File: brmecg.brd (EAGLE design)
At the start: 60.6 x 28.6 mm, 42 parts, among them U1 ADS1194CPAG

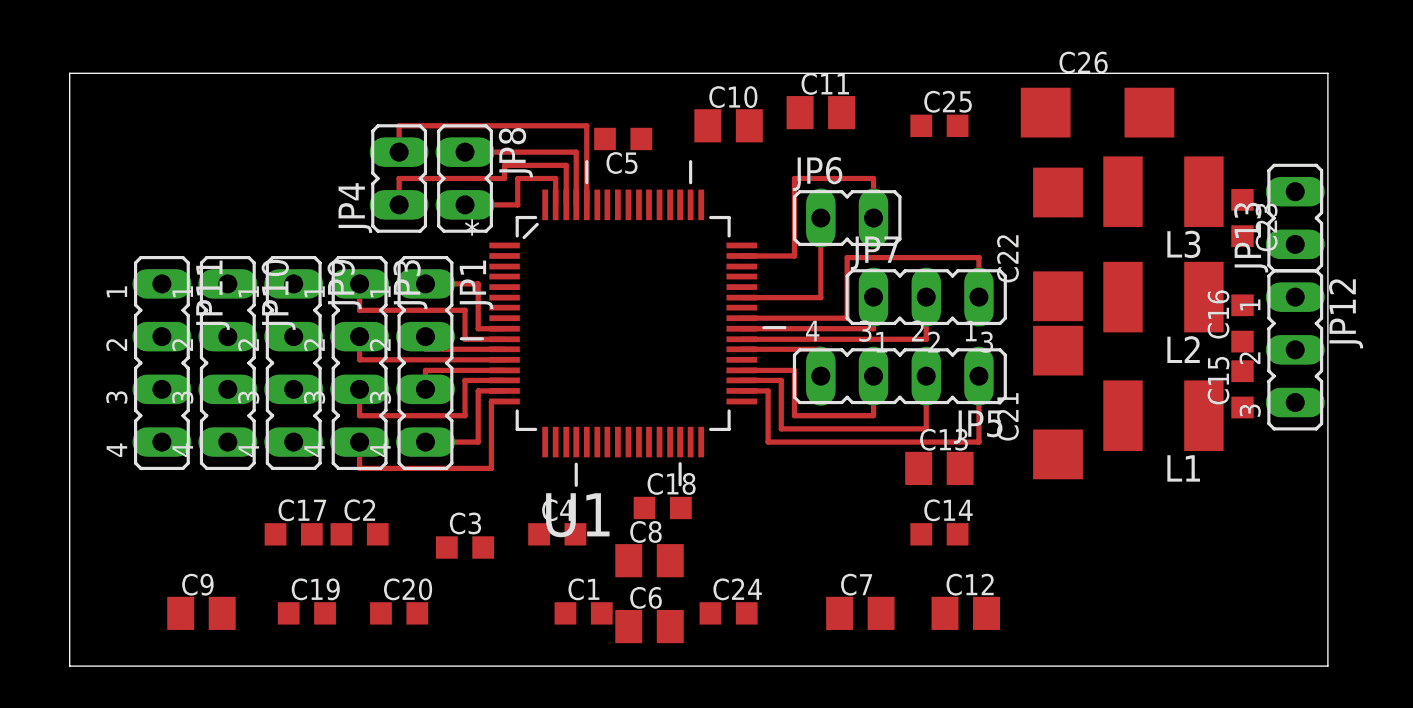
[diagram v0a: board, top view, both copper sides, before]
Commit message: Prepared for sex
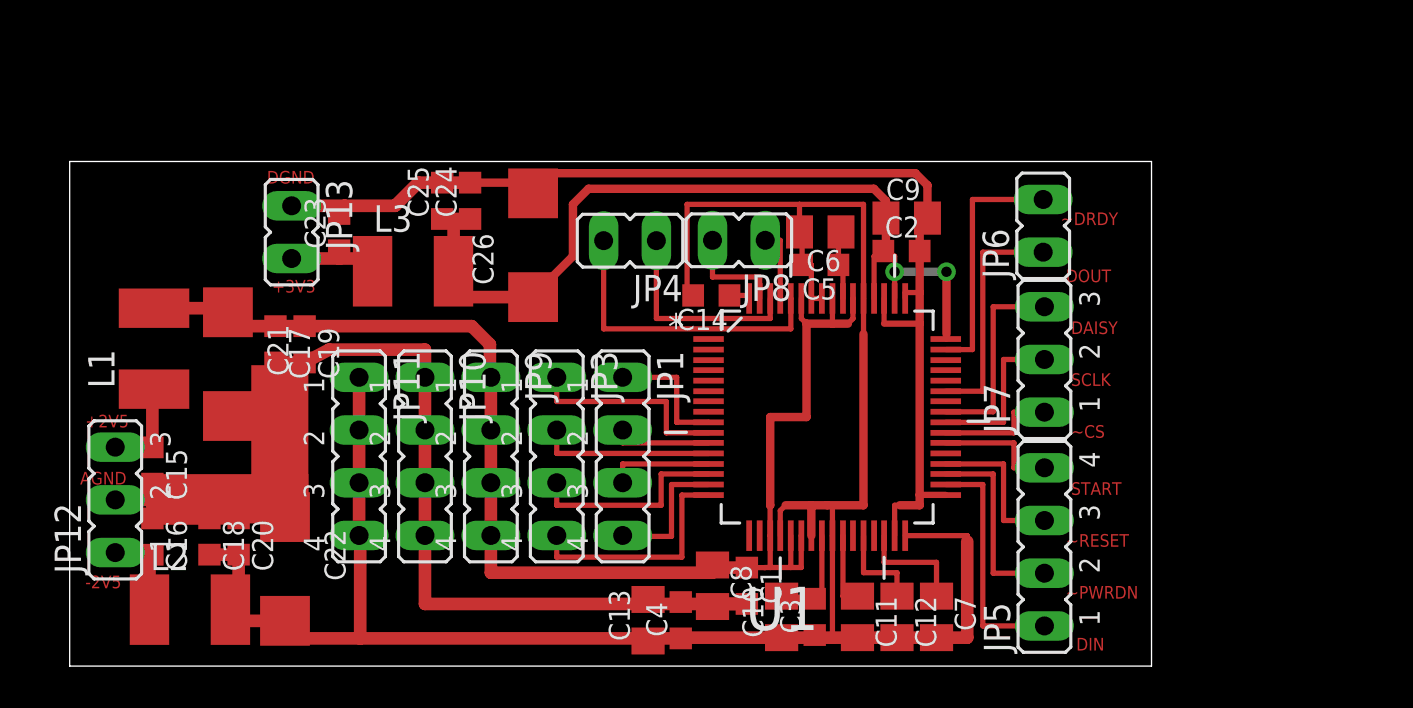
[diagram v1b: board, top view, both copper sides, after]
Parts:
- moved JP12 57.3 mm to (2.19, 8.01), turned to 90 degrees
- moved C16 53.5 mm to (3.98, 6.24), turned to 270 degrees
- moved C15 52.7 mm to (3.98, 9.66), turned to 270 degrees
- moved L2 49.3 mm to (5.79, 2.72), turned to 0 degrees
- moved L1 48.7 mm to (4.07, 15.3), turned to 90 degrees
- moved JP13 48.4 mm to (10.7, 20.9), turned to 180 degrees
- moved C23 43.5 mm to (13.0, 20.9), turned to 90 degrees
- moved C22 40.4 mm to (10.4, 4.68), turned to 270 degrees
- moved C21 40.0 mm to (7.62, 14.6), turned to 270 degrees
- moved C9 39.0 mm to (40.3, 21.6)
- moved L3 36.4 mm to (16.5, 19.0), turned to 0 degrees
- moved C2 29.5 mm to (40.1, 20.0)
- moved C26 27.9 mm to (22.3, 20.3), turned to 90 degrees
- moved C11 24.4 mm to (38.0, 2.37), turned to 270 degrees
- moved C25 24.2 mm to (17.9, 22.4), turned to 90 degrees
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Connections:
- net N$18 renamed DIN
- net N$19 renamed ~PWDN
- net N$20 renamed ~RESET
- net N$21 renamed START
- net N$23 renamed DAISY_IN
- net N$26 renamed DOUT
- net N$27 renamed ~DRDY
- removed net N$22: JP7.1, U1.40
- removed net N$25: JP7.2, U1.39
- new net SCLK: JP7.2, U1.40
- new net ~CS: JP7.1, U1.39
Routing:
- net -2V5: track 0.00 -> 109.4 mm
- net +2V5: track 0.00 -> 66.3 mm
- net AGND: track 0.00 -> 57.0 mm
- net GND: track 0.00 -> 56.7 mm
- net +3V3: track 0.00 -> 43.7 mm, vias 0 -> 2
- net N$25: track 10.9 -> 0.00 mm
- net N$22: track 7.87 -> 0.00 mm
- net SCLK: track 0.00 -> 7.78 mm
- net DAISY_IN: track 16.3 -> 9.82 mm
- net ~CS: track 0.00 -> 5.75 mm
- net DIN: track 17.1 -> 11.6 mm
- net N$3: track 0.00 -> 5.44 mm
- net N$1: track 0.00 -> 5.11 mm
- net +2V5/1: track 0.00 -> 4.69 mm
- net -2V5/1: track 0.00 -> 4.68 mm
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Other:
- board size 60.6 x 28.6 mm -> 52.1 x 24.3 mm
- board text added: "+2V5"
- board text added: "+3V3"
- board text added: "-2V5"
- board text added: "AGND"
- board text added: "DAISY"
- board text added: "DGND"
- board text added: "DIN"
- board text added: "DOUT"
- board text added: "SCLK"
- board text added: "START"
- board text added: "~CS"
- board text added: "~DRDY"
- board text added: "~PWRDN"
- board text added: "~RESET"
